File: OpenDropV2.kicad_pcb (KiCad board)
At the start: 2 copper layers, 100 x 100 mm, 200 parts, among them J1 DC_JACK, P1 CONN_01X01, P2 CONN_01X01, P3 CONN_01X01, P4 CONN_01X01, P5 CONN_01X01, Q1 BSS138, Q2 BSS138, Q3 BSS138, SW1 SW_PUSH, SW2 SW_PUSH, SW3 SW_PUSH, SW4 SW_PUSH, SW5 SPST, T1 IRF 840S, U1 MAX1771ESA, U2 HV507, U3 ARDUINO_MICRO, U4 HV507, U5 ESP8266_SMD

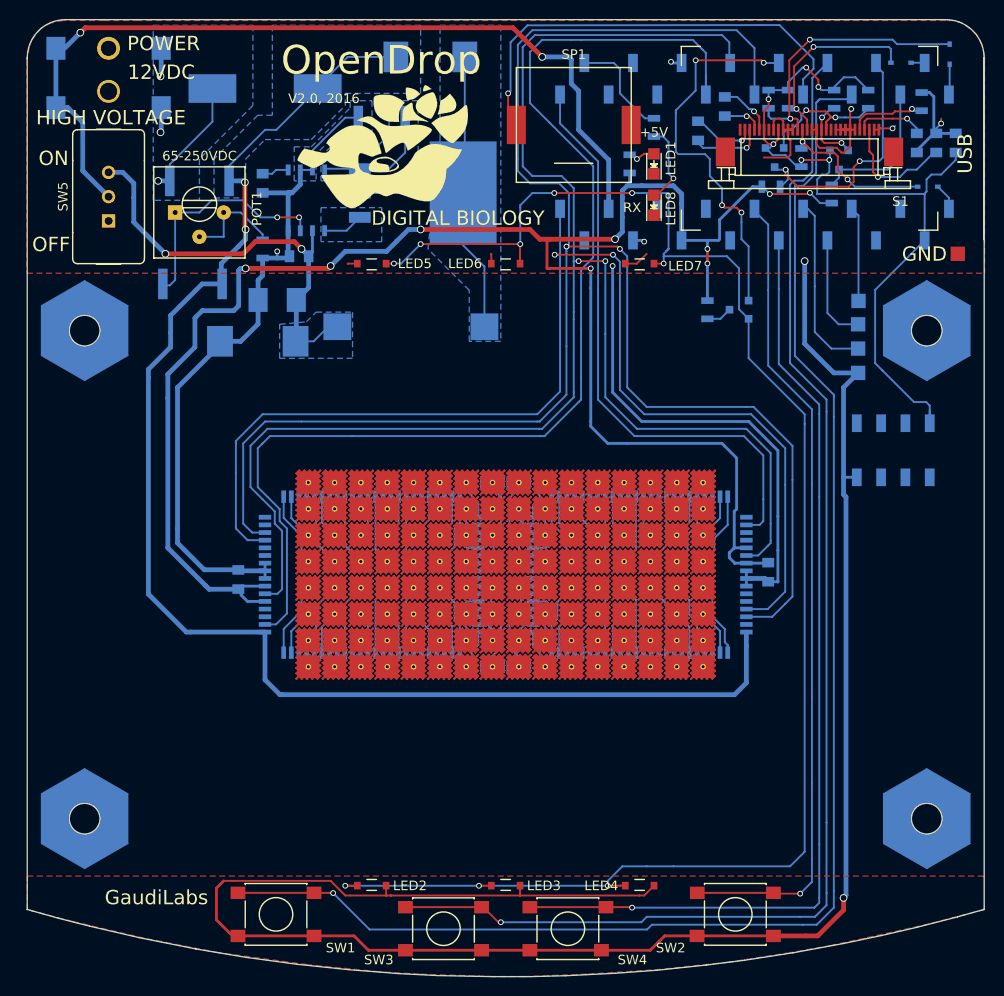
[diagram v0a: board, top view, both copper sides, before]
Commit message: started with corrections for V2.1
work in progress
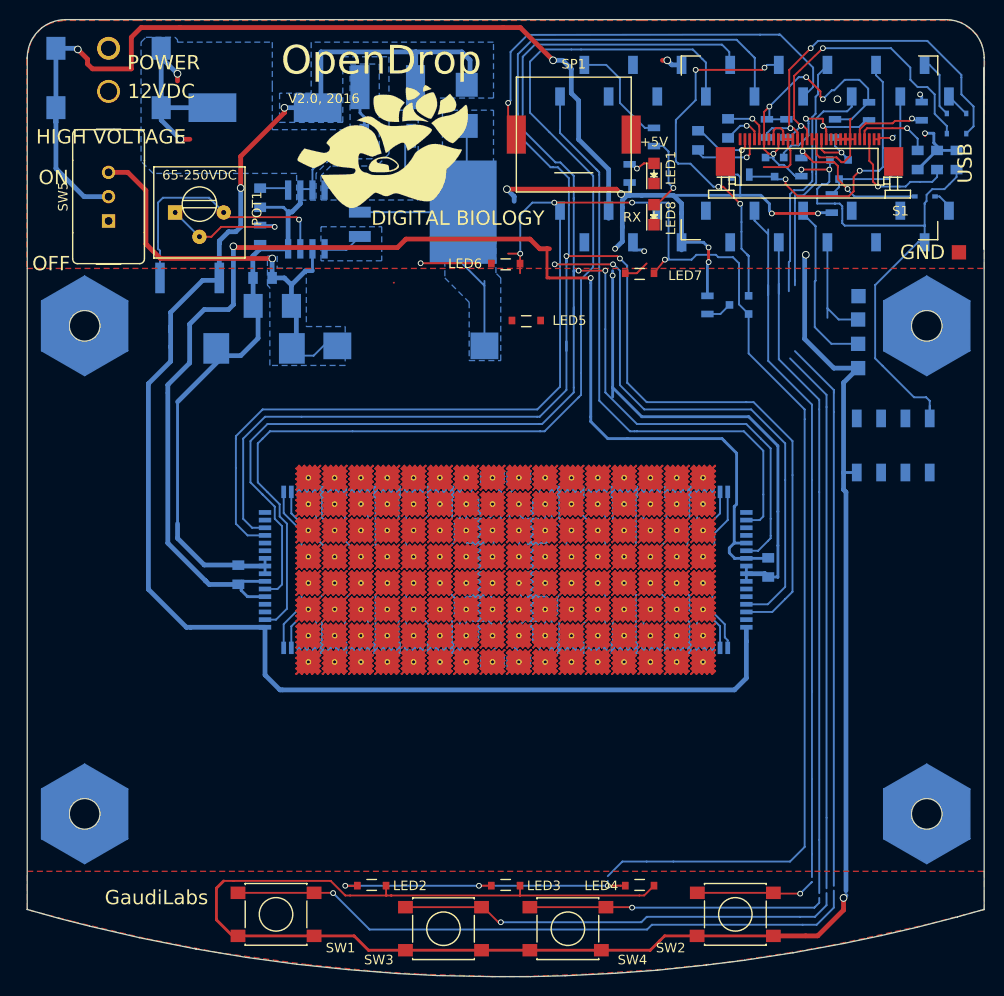
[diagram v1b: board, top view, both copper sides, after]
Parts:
- C6: footprint Resistors_SMD:R_2512 -> GaudiLabsFootPrints:C100n_250V
- D1: footprint Diodes_SMD:DO-214AB -> GaudiLabsFootPrints:DO-214AA
- D2, D3, D4: value D_Small -> 1N4148
- POT1: value POT -> 5k Ohm
- R5: value 390 -> 10
- U1: footprint SMD_Packages:SOIC-8-N -> GaudiLabsFootPrints:SO08
- moved C6 22.0 mm to (87.7, 49.1), turned to 0 degrees
- moved LED5 17.2 mm to (102.2, 73.4)
- moved D4 7.95 mm to (146.1, 52.9), turned to 270 degrees
- moved D2 7.45 mm to (148.1, 52.9), turned to 270 degrees
- moved D1 6.33 mm to (95.9, 51.0), turned to 90 degrees
- moved C2 4.44 mm to (74.6, 69.0)
- moved R8 3.46 mm to (124.5, 58.2)
- moved R14 3.06 mm to (129.3, 53.4)
- moved R11 3.06 mm to (127.3, 53.4)
- moved R13 3.05 mm to (134.4, 53.4)
- moved C9 2.31 mm to (123.2, 53.4)
- moved C4 2.00 mm to (74.9, 51.2)
- moved L1 2.00 mm to (90.1, 76.1)
- moved T1 2.00 mm to (84.8, 62.1)
- moved U1 2.00 mm to (79.2, 62.9)
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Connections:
- POT1 pad 1: V_READ_HV -> Net-(POT1-Pad1)
- POT1 pad 2: Net-(POT1-Pad2) -> Net-(POT1-Pad1)
- POT1 pad 3: Net-(POT1-Pad2) -> V_READ_HV
- R1 pad 1: Net-(POT1-Pad2) -> Net-(POT1-Pad1)
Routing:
- net (no net): track 0.02 -> 269.8 mm, vias 0 -> 3
- net SW2: track 85.3 -> 14.8 mm
- net SW1: track 157.1 -> 91.5 mm
- net SW4: track 101.4 -> 36.0 mm
- net SW3: track 137.8 -> 72.6 mm
- net V_HV: track 149.7 -> 165.5 mm
- net Net-(LED2-Pad2): track 172.4 -> 157.9 mm, vias 9 -> 7
- net Net-(POT1-Pad1): track 0.00 -> 13.5 mm, vias 0 -> 1
- net GND: track 381.1 -> 368.7 mm, vias 12 -> 9
- net Net-(D4-Pad2): track 20.6 -> 32.6 mm
- net Net-(POT1-Pad2): track 10.7 -> 0.00 mm
- net Net-(D2-Pad2): track 29.1 -> 39.2 mm
- net Net-(P1-Pad1): track 9.92 -> 0.00 mm
- net +5V: track 193.5 -> 202.5 mm
- net 3.3V: track 85.8 -> 94.1 mm
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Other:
- outline, holes or cut-outs redrawn
